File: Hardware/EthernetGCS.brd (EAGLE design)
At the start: 72.4 x 45.3 mm, 80 parts, among them IC1 PIC24FJ64GA002_QFN, IC3 24AA00OT, J2 HR911105A, Q2 25Mhz, U1 MIC5219-3.3V, U3 MIC5219-3.3V, U4 ENC28J60-QFN, U5 MIC5219-3.3V, U7 FT232RL-BASICSSOP, X2 USB-A-H

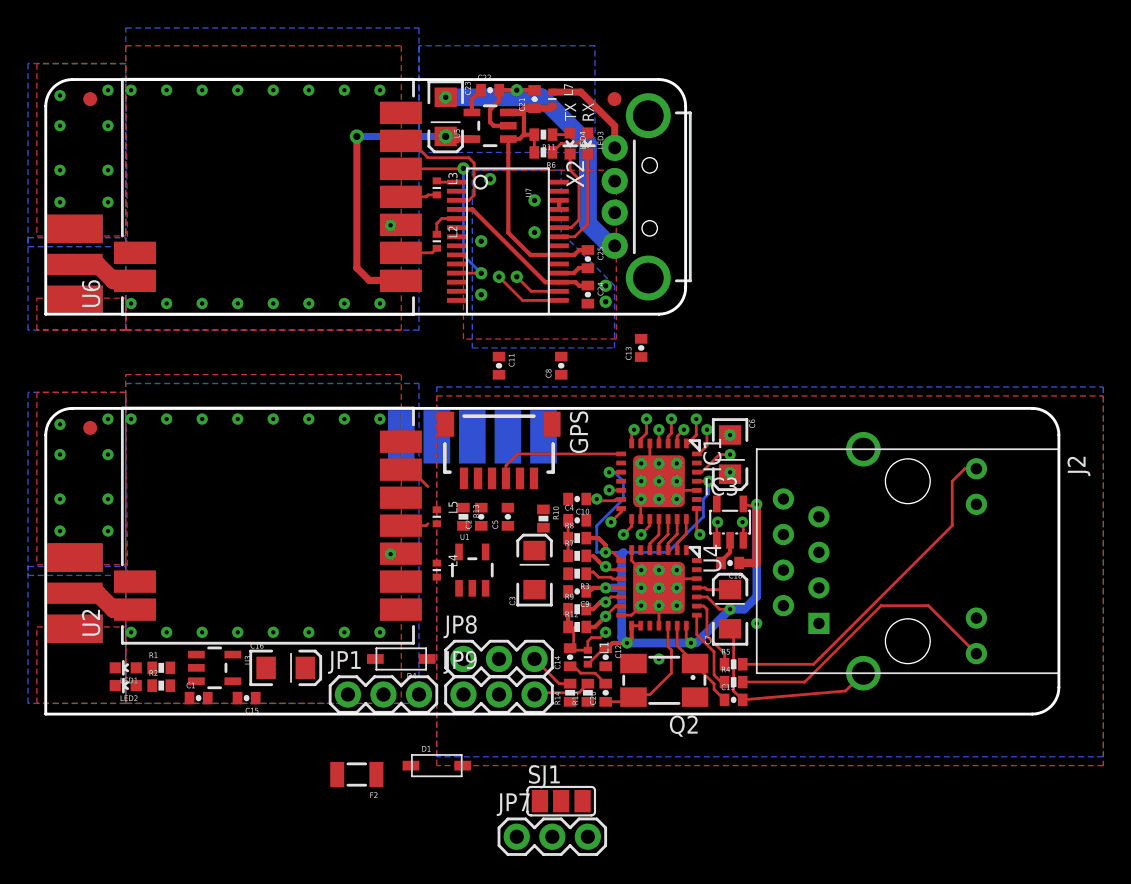
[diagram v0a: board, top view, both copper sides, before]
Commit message: More Layout...
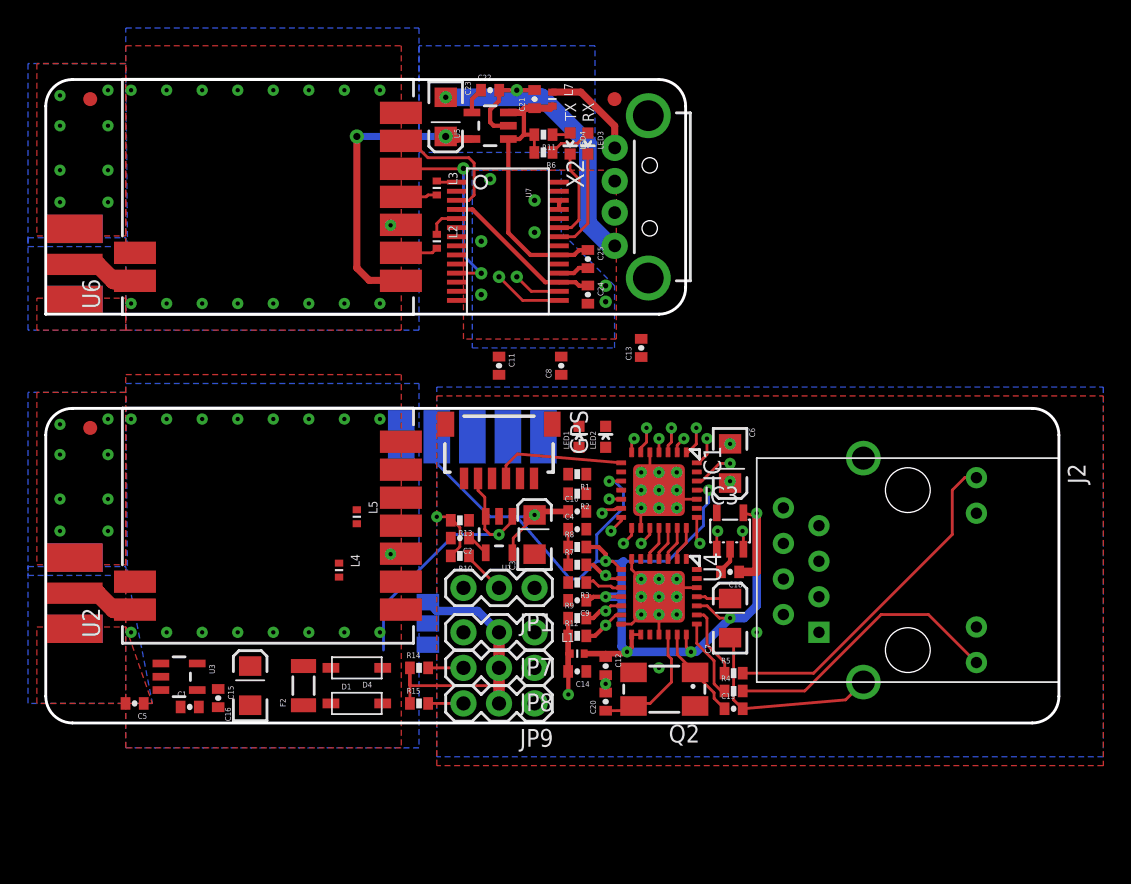
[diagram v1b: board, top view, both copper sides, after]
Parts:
- moved LED2 38.6 mm to (40.0, 19.7), turned to 0 degrees
- moved LED1 36.4 mm to (38.1, 19.7), turned to 0 degrees
- moved R1 32.8 mm to (38.0, 17.0), turned to 180 degrees
- moved R2 32.7 mm to (38.0, 15.6), turned to 180 degrees
- moved C5 29.8 mm to (6.35, 0.64), turned to 180 degrees
- moved SJ1 15.9 mm to (27.3, 6.35), flipped to the bottom, turned to 270 degrees
- moved JP1 15.4 mm to (34.9, 8.89), turned to 180 degrees
- moved JP7 14.7 mm to (34.9, 5.71), turned to 180 degrees
- moved R15 12.1 mm to (26.7, 0.64), turned to 0 degrees
- moved R14 10.9 mm to (26.7, 3.17), turned to 0 degrees
- moved F2 7.41 mm to (18.4, 1.91), turned to 90 degrees
- moved D1 7.24 mm to (22.2, 0.64)
- moved L4 6.99 mm to (21.0, 10.2)
- moved R10 6.54 mm to (29.6, 11.2), turned to 180 degrees
- moved L5 5.71 mm to (22.2, 14.0)
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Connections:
- net 5V: now also GPS.5
- net V+: no longer GPS.5
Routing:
- net V+: track 65.6 -> 90.2 mm, vias 7 -> 8
- net V_RC: track 0.00 -> 21.6 mm
- net 5V: track 22.5 -> 42.7 mm, vias 0 -> 1
- net BAT_SEN: track 14.0 -> 26.5 mm, vias 1 -> 2
- net RC2: track 18.3 -> 26.8 mm
- net RC1: track 18.2 -> 26.0 mm
- net N$11: track 0.00 -> 3.17 mm
- net GND: track 67.3 -> 64.2 mm, vias 80 -> 81
- net N$7: track 1.99 -> 0.00 mm
- net N$2: track 0.00 -> 1.63 mm
- net RTS: track 23.6 -> 22.0 mm
- net SCL: track 10.5 -> 11.6 mm
- net SDA: track 12.7 -> 13.7 mm
- net RD+: track 20.0 -> 20.7 mm
- net PGD: track 16.2 -> 15.6 mm
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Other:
- board size 72.4 x 45.3 mm -> 72.4 x 46 mm
